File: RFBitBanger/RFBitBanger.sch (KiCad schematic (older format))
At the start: 82 parts, among them J1 POWER, J10 Conn_01x04, J11 SPEAKER, J13 Conn_01x01, J14 Conn_01x01, J15 Conn_01x01, J16 Conn_01x01, J2 Barrel_Jack, J3 Conn_01x01, J4 Conn_01x01, J5 Conn_01x04, J6 Conn_01x01, J7 Conn_01x01, J8 Conn_01x01, J9 ICSP, P1 Mini-DIN_6pins_ver4, Q14 2N3904, Q4 2N3904, SW1 SW_Push, SW2 SW_Push, SW3 SW_Push, SW4 SW_Push, SW5 SW_Push, T4 Common-Mode Choke, U1 ATMEGA328-PU, U2 LM7805_TO220, U3 LM386, U5 LCD-016N002L, Y1 16 MHz

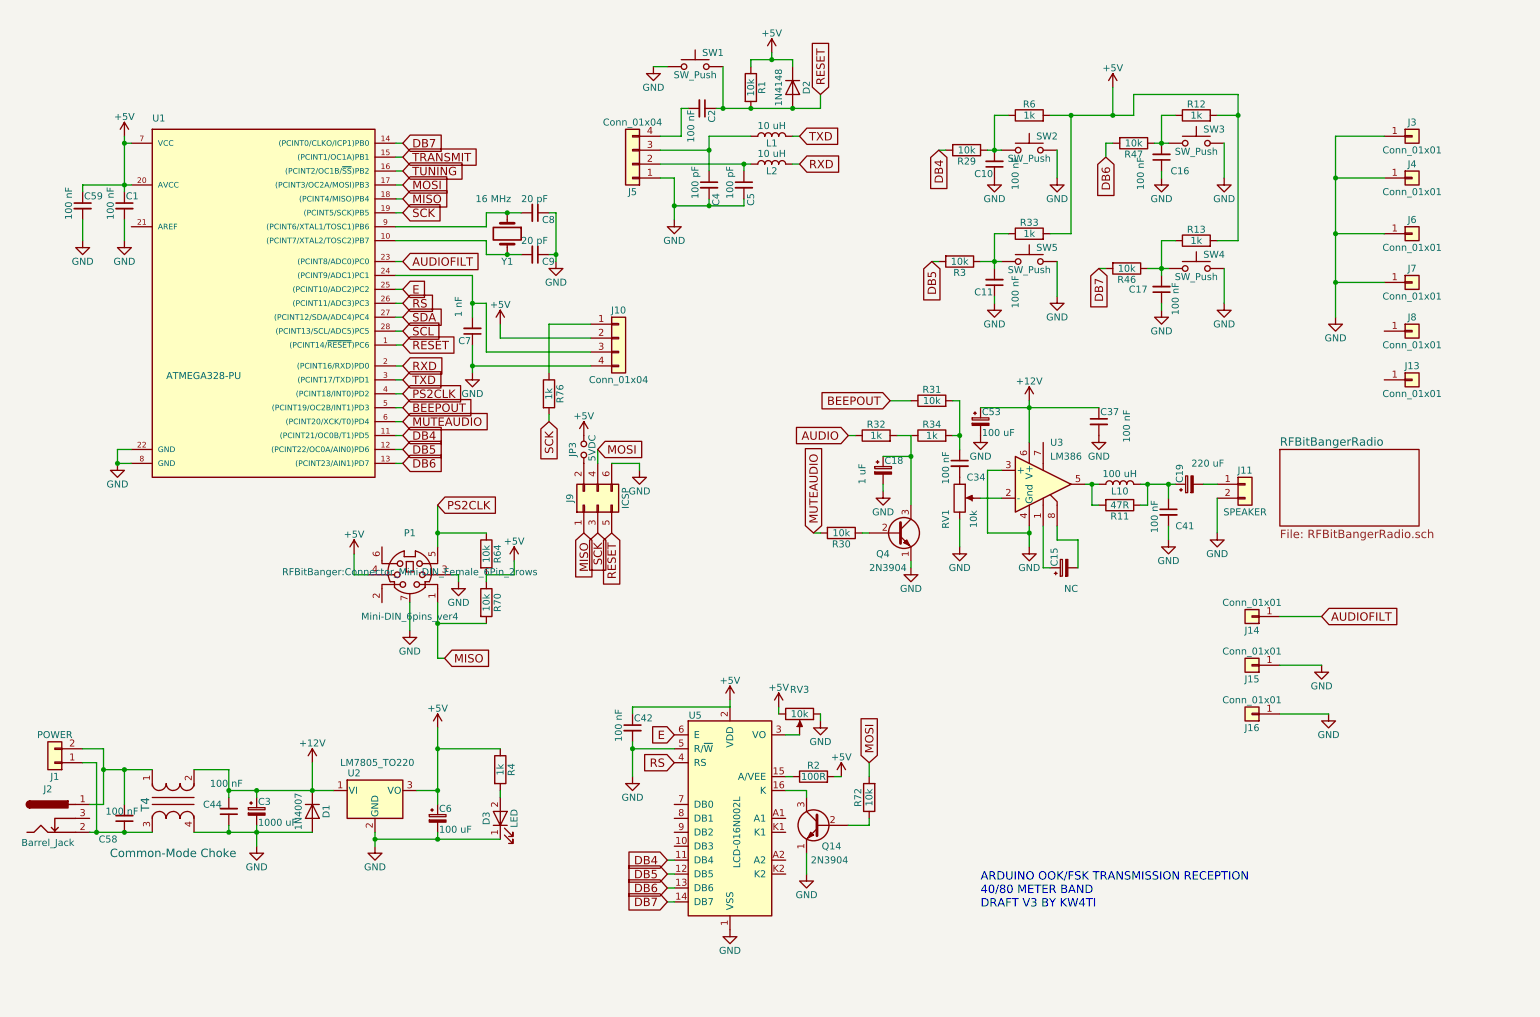
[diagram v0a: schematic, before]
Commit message: Implemented timers, fixed beep audio, fixed key shaping
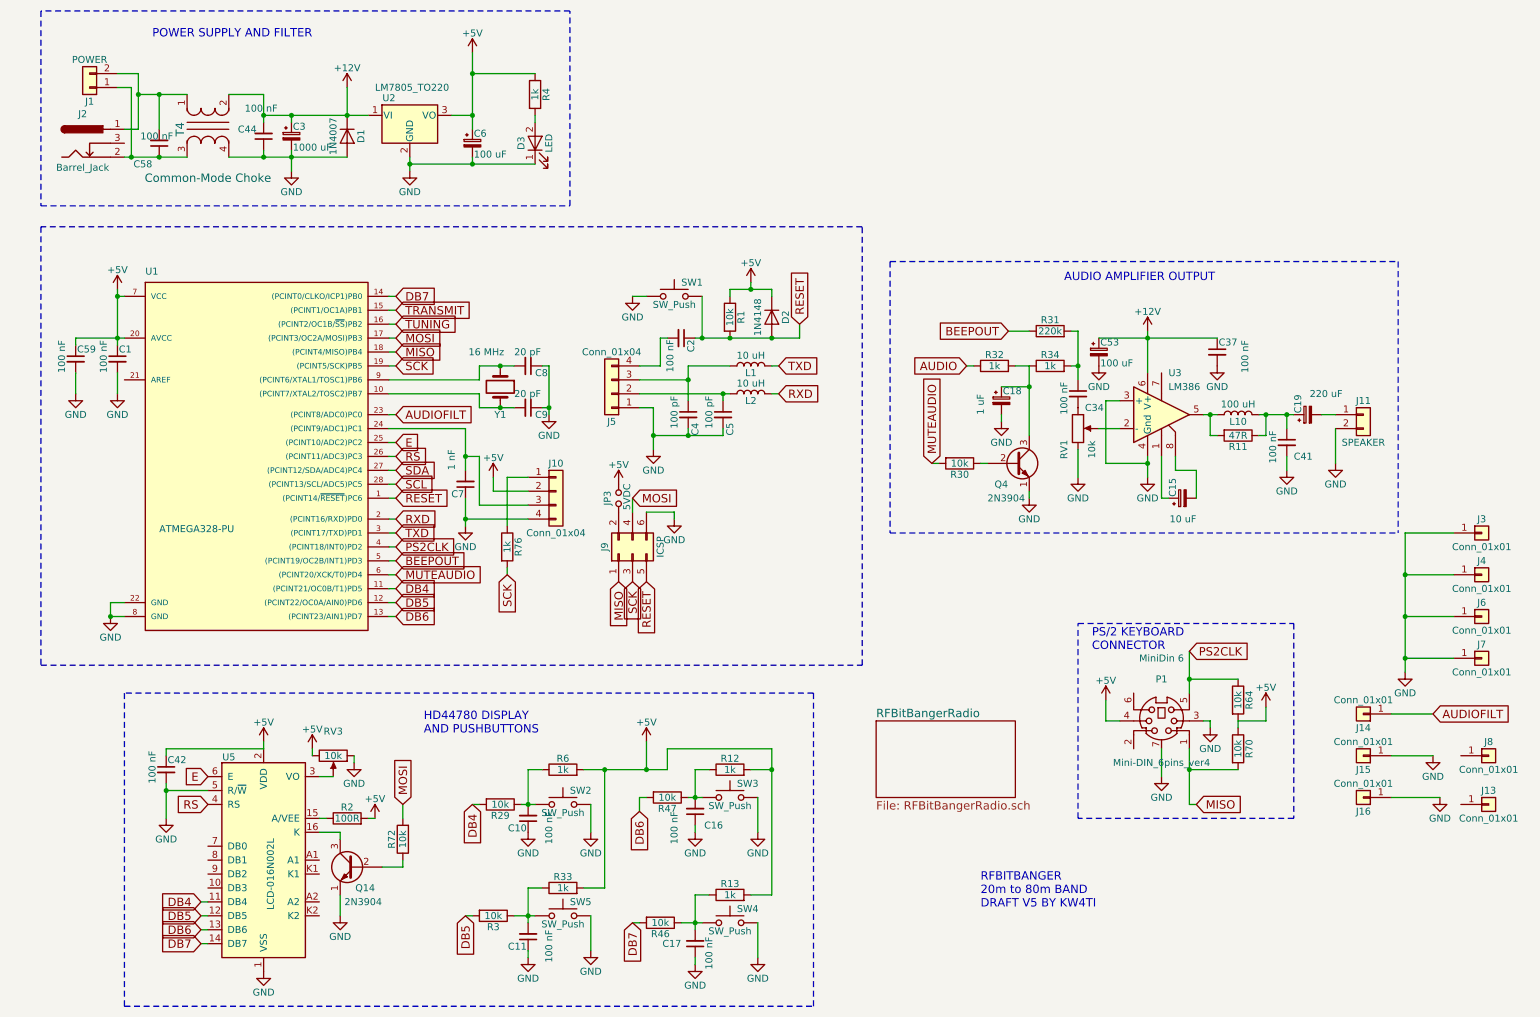
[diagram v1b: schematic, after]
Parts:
- C15: value NC -> 10 uF
- P1: footprint RFBitBanger:Connector_Mini-DIN_Female_6Pin_2rows -> MiniDin 6
- R31: value 10k -> 220k
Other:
- note added: "AUDIO AMPLIFIER OUTPUT"
- note added: "HD44780 DISPLAY\nAND PUSHBUTTONS"
- note added: "POWER SUPPLY AND FILTER"
- note added: "PS/2 KEYBOARD\nCONNECTOR"
- note added: "RFBITBANGER\n20m to 80m BAND\nDRAFT V5 BY KW4TI"
- note removed: "ARDUINO OOK/FSK TRANSMISSION RECEPTION\n40/80 METER BAND\nDRAFT V3 BY KW4TI"
- moved on the sheet: C1, C10, C11, C15, C16, C17, C18, C19, C2, C3, C34, C37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
